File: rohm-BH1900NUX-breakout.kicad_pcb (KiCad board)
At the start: 2 copper layers, 7.9 x 18.3 mm, 11 parts, among them J1 Conn_01x04_Socket, U1 BH1900NUX-TR

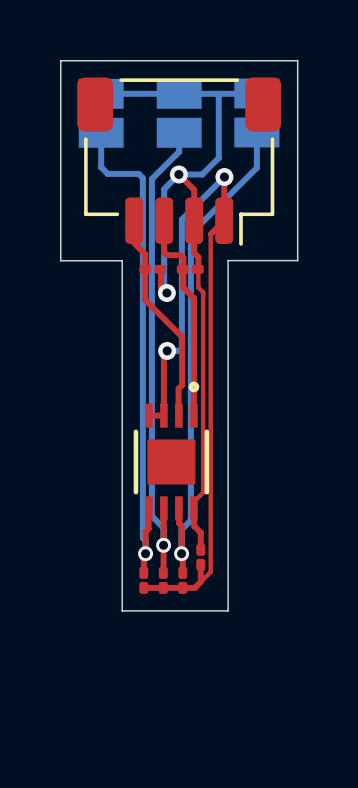
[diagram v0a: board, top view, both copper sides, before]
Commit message: Layout updated
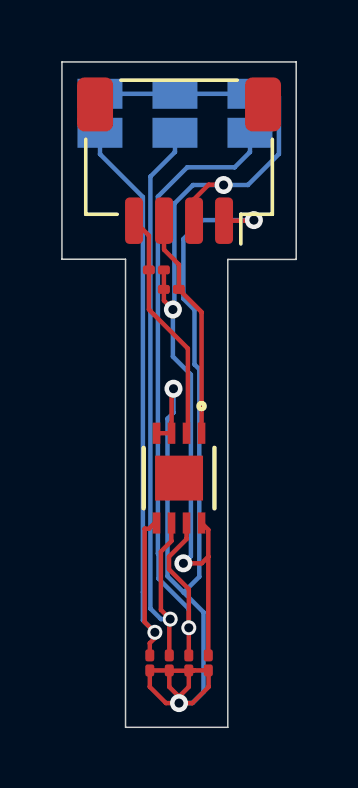
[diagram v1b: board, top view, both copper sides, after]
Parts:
- J1: footprint Connector_JST:JST_SH_SM04B-SRSS-TB_1x04-1MP_P1.00mm_Horizontal -> Riehlhome:JST_SH_SM04B-SRSS-TB_1x04-1MP_P1.00mm_Horizontal
- U1: footprint Rohm_BH1900NUX_ALT:VSON008X2030_ROM-M -> Rohm_BH1900NUX_ALT:VSON008X2030_ROM
- moved C1 3.53 mm to (136.5, 96.7)
- moved R1 2.76 mm to (134.5, 96.7)
- moved R4 2.76 mm to (135.2, 96.7)
- moved R5 2.76 mm to (135.8, 96.7)
- moved R3 0.92 mm to (135.2, 84.3), turned to 0 degrees
- moved U1 0.59 mm to (135.5, 90.6)
- moved JP3 0.23 mm to (137.9, 78.4)
- moved JP2 0.14 mm to (135.4, 78.4)
- moved R2 0.12 mm to (134.7, 83.6)
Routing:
- net GND: track 26.7 -> 37.2 mm, vias 2 -> 3
- net Net-(JP3-B): track 17.3 -> 24.1 mm
- net +3V3: track 28.0 -> 33.7 mm, vias 2 -> 3
- net Net-(JP2-B): track 16.5 -> 21.7 mm
- net Net-(JP1-A): track 17.7 -> 22.3 mm
- net SCL: track 7.24 -> 7.88 mm
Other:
- board size 7.9 x 18.3 mm -> 7.8 x 22.2 mm
